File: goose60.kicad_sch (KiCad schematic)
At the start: 32 parts, among them SW1 SW_Push, SW2 SW_Push, U1 STM32F103CBTx, X1 Crystal_GND24

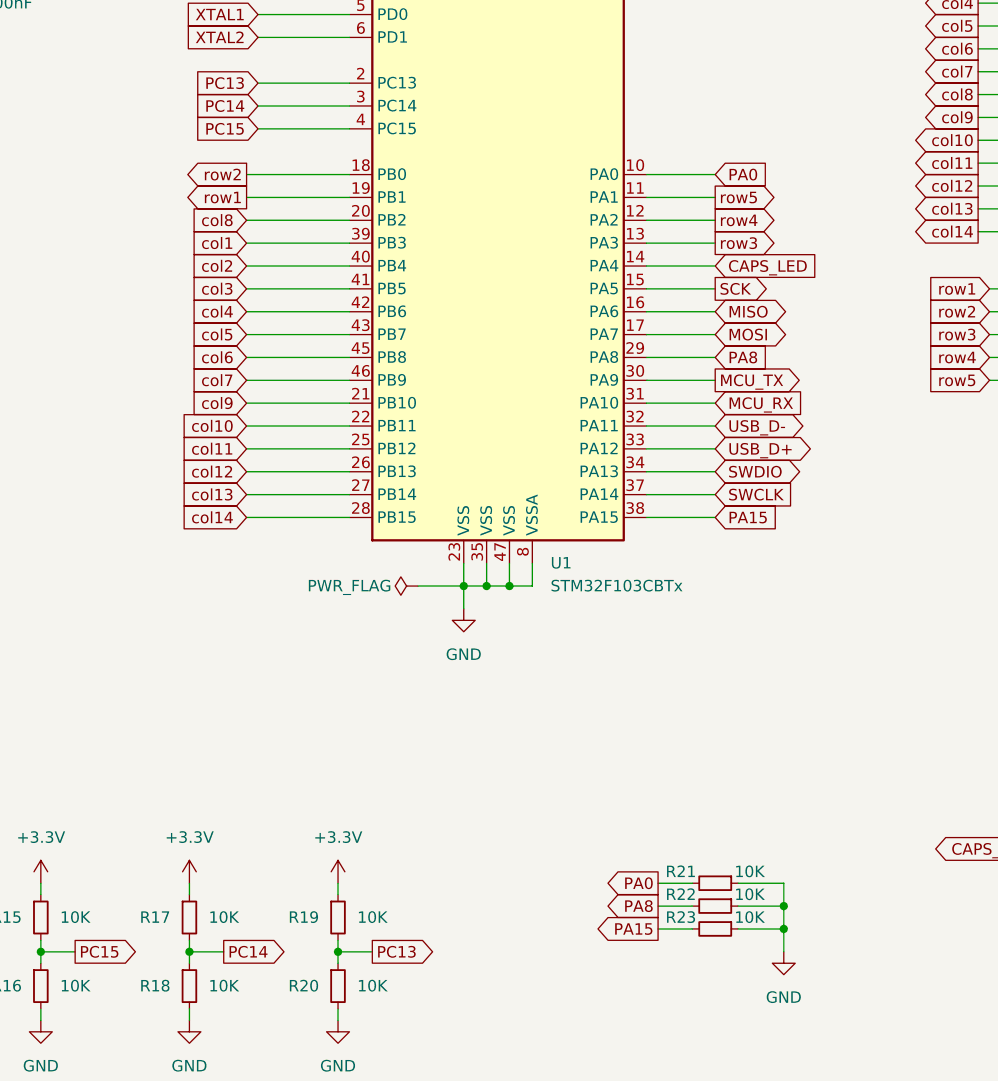
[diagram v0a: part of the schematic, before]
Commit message: change pin default and try layout
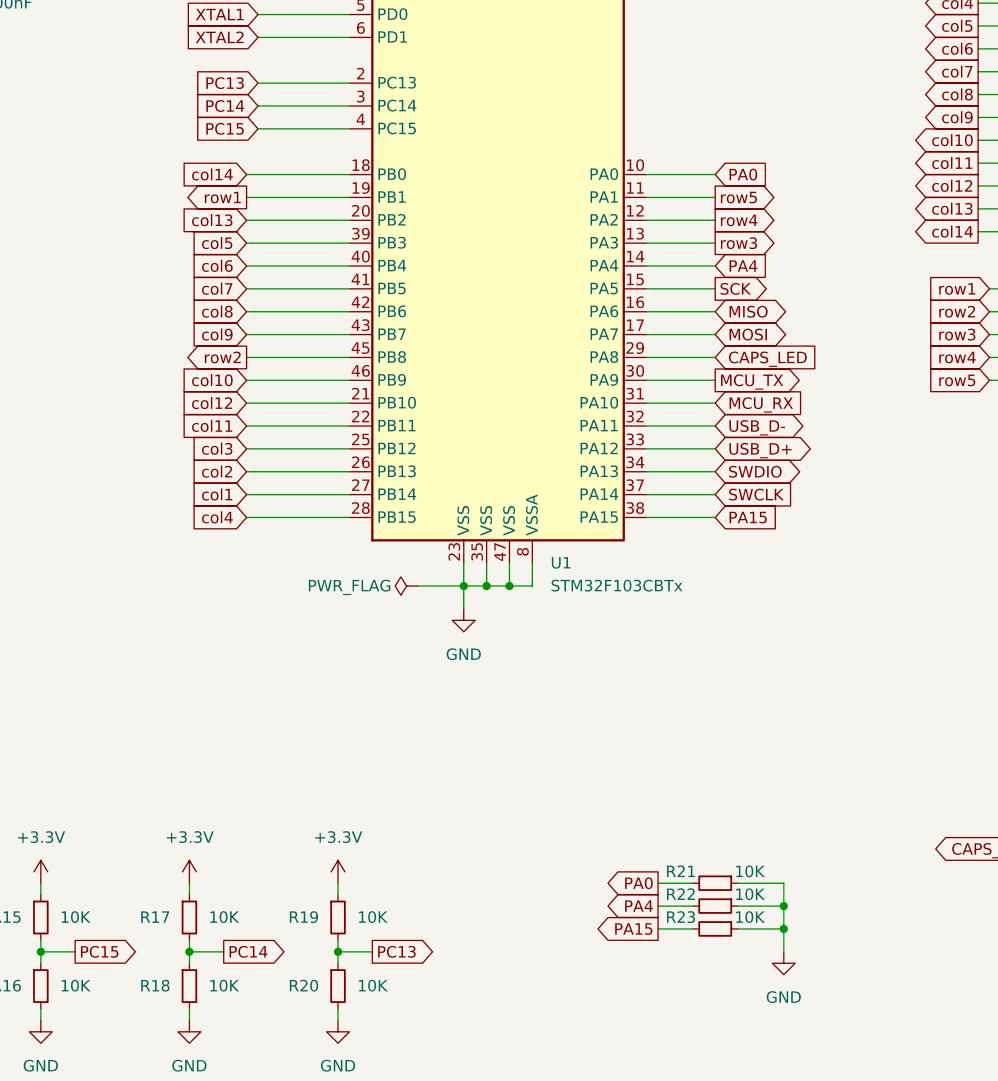
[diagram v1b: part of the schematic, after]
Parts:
- H2, H3, H5, H6: footprint MountingHole:MountingHole_3.2mm_M3_Pad -> MountingHole:MountingHole_3.2mm_M3_Pad_TopOnly
- H4: footprint MountingHole:MountingHole_3.2mm_M3 -> MountingHole:MountingHole_3.2mm_M3_Pad_TopOnly
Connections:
- net CAPS_LED: now also U1.29 (PA8); no longer U1.14 (PA4)
- net col1: now also U1.27 (PB14); no longer U1.39 (PB3)
- net col10: now also U1.46 (PB9); no longer U1.22 (PB11)
- net col11: now also U1.22 (PB11); no longer U1.25 (PB12)
- net col12: now also U1.21 (PB10); no longer U1.26 (PB13)
- net col13: now also U1.20 (PB2); no longer U1.27 (PB14)
- net col14: now also U1.18 (PB0); no longer U1.28 (PB15)
- net col2: now also U1.26 (PB13); no longer U1.40 (PB4)
- net col3: now also U1.25 (PB12); no longer U1.41 (PB5)
- net col4: now also U1.28 (PB15); no longer U1.42 (PB6)
- net col5: now also U1.39 (PB3); no longer U1.43 (PB7)
- net col6: now also U1.40 (PB4); no longer U1.45 (PB8)
- net col7: now also U1.41 (PB5); no longer U1.46 (PB9)
- net col8: now also U1.42 (PB6); no longer U1.20 (PB2)
- net col9: now also U1.43 (PB7); no longer U1.21 (PB10)
- net row2: now also U1.45 (PB8); no longer U1.18 (PB0)
- net PA8 renamed PA4
- net PA4: now also U1.14 (PA4); no longer U1.29 (PA8)
